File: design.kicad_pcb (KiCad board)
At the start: 2 copper layers, 28.5 x 12 mm, 7 parts, among them J1 USB_C_Receptacle, J2 Conn_01x05, U1 ATtiny1616-M

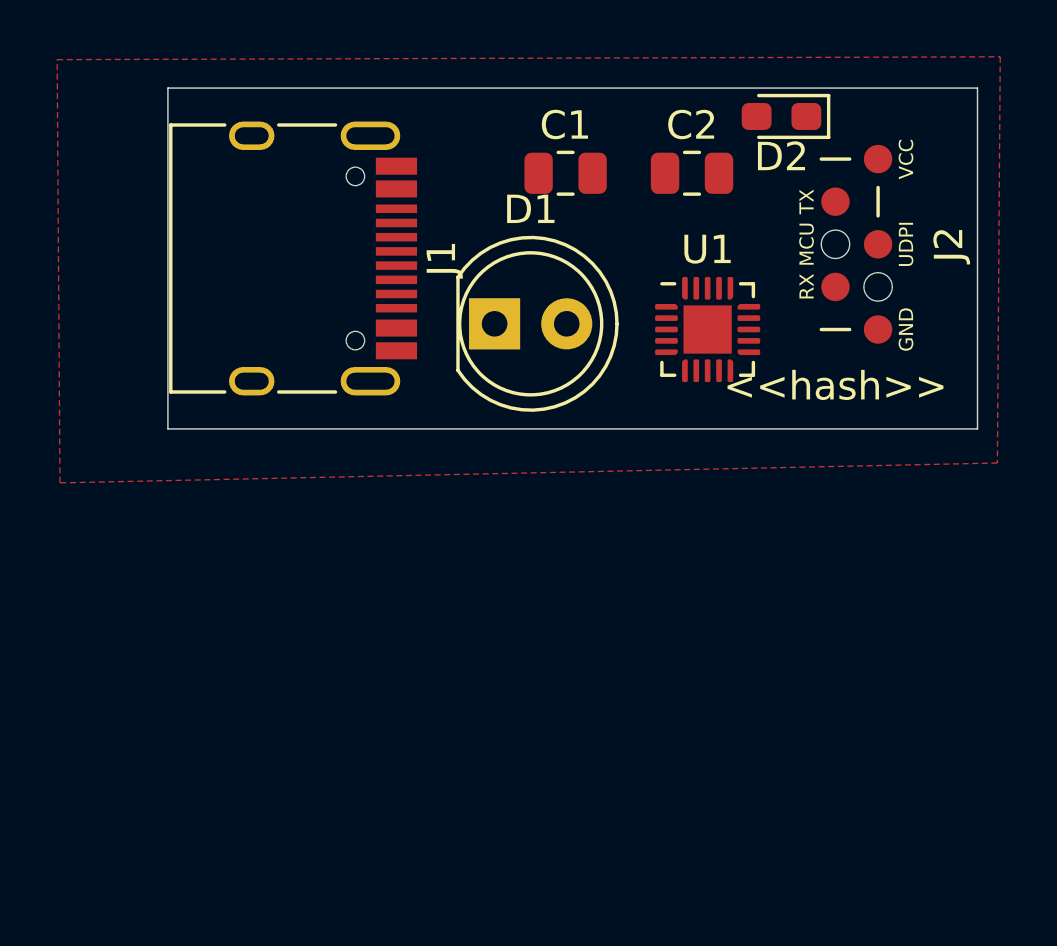
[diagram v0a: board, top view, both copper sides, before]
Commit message: Moved to KiCad V6
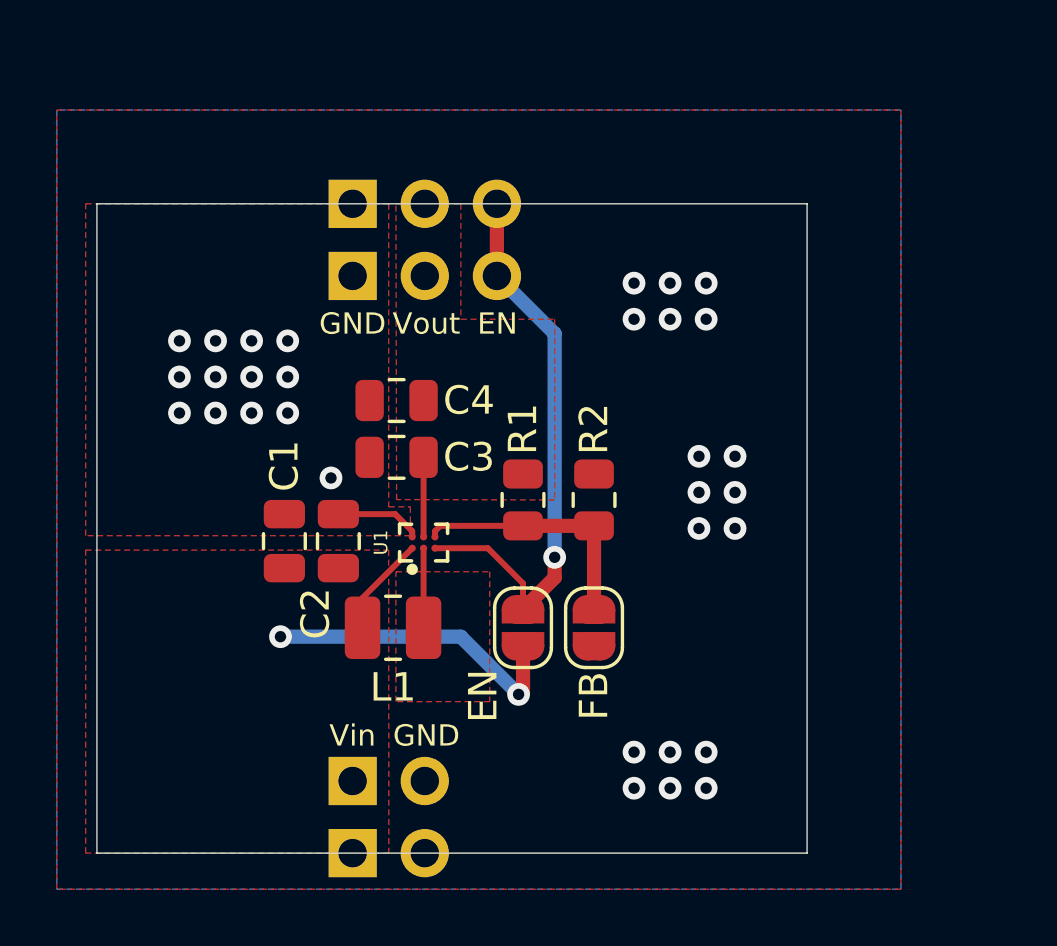
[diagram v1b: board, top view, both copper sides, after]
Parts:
- removed D1: LED, LED_THT:LED_D5.0mm_FlatTop
- removed D2: LED, LED_SMD:LED_0603_1608Metric_Pad1.05x0.95mm_HandSolder
- added C3: C_Small, Capacitor_SMD:C_0805_2012Metric, F.Cu at (144.6, 93.0)
- added C4: C_Small, Capacitor_SMD:C_0805_2012Metric, F.Cu at (144.6, 91.0)
- added J3: Conn_01x03, Connector_PinHeader_2.54mm:PinHeader_1x03_P2.54mm_Vertical, F.Cu at (143.0, 86.6)
- added J4: Conn_01x03, Connector_PinHeader_2.54mm:PinHeader_1x03_P2.54mm_Vertical, F.Cu at (143.0, 84.1)
- added JP1: SolderJumper_2_Open, Jumper:SolderJumper-2_P1.3mm_Open_RoundedPad1.0x1.5mm, F.Cu at (149.0, 99.0)
- added JP2: SolderJumper_2_Open, Jumper:SolderJumper-2_P1.3mm_Open_RoundedPad1.0x1.5mm, F.Cu at (151.5, 99.0)
- added L1: L_Small, Inductor_SMD:L_1008_2520Metric, F.Cu at (144.4, 99.0)
- added R1: R_Small, Resistor_SMD:R_0805_2012Metric, F.Cu at (149.0, 94.5)
- added R2: R_Small, Resistor_SMD:R_0805_2012Metric, F.Cu at (151.5, 94.5)
- J1: value USB_C_Receptacle -> Conn_01x02; footprint Connector_USB:USB_C_Receptacle_HRO_TYPE-C-31-M-12 -> Connector_PinHeader_2.54mm:PinHeader_1x02_P2.54mm_Vertical
- J2: value Conn_01x05 -> Conn_01x02; footprint E32-xxxT20D:UDPI_interface -> Connector_PinHeader_2.54mm:PinHeader_1x02_P2.54mm_Vertical
- U1: value ATtiny1616-M -> TPS61099YFFT; footprint Package_DFN_QFN:VQFN-20-1EP_3x3mm_P0.4mm_EP1.7x1.7mm -> Converter_DCDC_custom:BGA6N40P3X2_122X88X62N
- moved J2 28.3 mm to (143.0, 106.9), turned to 90 degrees
- moved J1 18.6 mm to (143.0, 104.4), turned to 90 degrees
- moved C2 18.0 mm to (142.5, 96.0), turned to 90 degrees
- moved C1 16.3 mm to (140.6, 96.0), turned to 90 degrees
- moved U1 12.5 mm to (145.5, 96.0), turned to 90 degrees
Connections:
- C1 pad 1: Net-(C1-Pad1) -> Vin
- C1 pad 2: Net-(C1-Pad2) -> GND
- C2 pad 1: Net-(C2-Pad1) -> Vin
- C2 pad 2: Net-(C2-Pad2) -> GND
- J2 pad 1: Net-(J2-Pad1) -> Vin
- J2 pad 2: Net-(J2-Pad2) -> GND
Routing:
- net En: track 0.00 -> 19.9 mm, vias 0 -> 1
- net Vin: track 0.00 -> 14.5 mm, vias 0 -> 2
- net FB: track 0.00 -> 8.82 mm
- net GND: track 0.00 -> 3.05 mm, vias 0 -> 31
- net Vout: track 0.00 -> 2.80 mm
- net SW: track 0.00 -> 2.80 mm
- added copper zone on B.Cu, net GND
- added copper zone on F.Cu, net GND
- added copper zone on F.Cu, net SW
- added copper zone on F.Cu, net Vin
- added copper zone on F.Cu, net Vout
- removed copper zone on F.Cu, net Net-(J1-PadA1)
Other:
- board size 28.5 x 12 mm -> 25 x 22.9 mm
- net class Default removed
- board text added: "<<project_name>> <<ID>> <<version>> <<date>> <<hash>> gll.wf/p/001"
- board text added: "EN"
- board text added: "GND"
- board text added: "Vin"
- board text added: "Vout"
- board text removed: "<<ID>>"
- board text removed: "<<date>>"
- board text removed: "<<hash>>"
- board text removed: "<<project_name>>"
- board text removed: "<<version>>"
